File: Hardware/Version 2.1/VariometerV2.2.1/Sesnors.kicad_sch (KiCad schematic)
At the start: 19 parts, among them U4 DPS310, U5 BMI088, U6 QMC5883L, U7 MAX98357A

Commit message: Working on PCB
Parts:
- R36: footprint (none) -> Resistor_SMD:R_0603_1608Metric
- R41: footprint (none) -> Resistor_SMD:R_0805_2012Metric
- TP7, TP8, TP9: footprint (none) -> TestPoint:TestPoint_Pad_D1.5mm
- U4: footprint (none) -> MainLibrary:DPS310XTSA1
- U5: footprint (none) -> MainLibrary:BMI088
- U6: footprint (none) -> MainLibrary:QMC5883L
- U7: footprint (none) -> MainLibrary:QFN50P300X300X80-17N
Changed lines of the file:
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@@
       (effects (font (size 1.27 1.27)) (justify left))
     )
-    (property "Footprint" "" (at 71.12 143.51 0)
+    (property "Footprint" "TestPoint:TestPoint_Pad_D1.5mm" (at 71.12 143.51 0)
       (effects (font (size 1.27 1.27)) hide)
     )
@@
       (effects (font (size 1.27 1.27)))
     )
-    (property "Footprint" "" (at 60.96 52.07 0)
+    (property "Footprint" "MainLibrary:BMI088" (at 60.96 52.07 0)
       (effects (font (size 1.27 1.27)) hide)
     )
@@
       (effects (font (size 1.27 1.27)) (justify left))
     )
-    (property "Footprint" "" (at 66.04 143.51 0)
+    (property "Footprint" "TestPoint:TestPoint_Pad_D1.5mm" (at 66.04 143.51 0)
       (effects (font (size 1.27 1.27)) hide)
     )
@@
       (effects (font (size 1.27 1.27)) (justify left))
     )
-    (property "Footprint" "" (at 137.16 49.53 0)
+    (property "Footprint" "MainLibrary:QMC5883L" (at 137.16 49.53 0)
       (effects (font (size 1.27 1.27)) hide)
     )
@@
       (effects (font (size 1.27 1.27)))
     )
-    (property "Footprint" "" (at 231.14 39.37 0)
+    (property "Footprint" "MainLibrary:DPS310XTSA1" (at 231.14 39.37 0)
       (effects (font (size 1.27 1.27)) hide)
     )
@@
       (effects (font (size 1.27 1.27)) (justify left))
     )
-    (property "Footprint" "" (at 62.23 143.51 0)
+    (property "Footprint" "TestPoint:TestPoint_Pad_D1.5mm" (at 62.23 143.51 0)
       (effects (font (size 1.27 1.27)) hide)
     )
@@
       (effects (font (size 1.27 1.27)) (justify left))
     )
-    (property "Footprint" "" (at 31.75 157.48 0)
+    (property "Footprint" "Resistor_SMD:R_0805_2012Metric" (at 31.75 157.48 0)
       (effects (font (size 1.27 1.27)) hide)
     )
@@
       (effects (font (size 1.27 1.27)) (justify left))
     )
-    (property "Footprint" "" (at 214.63 44.45 0)
+    (property "Footprint" "Resistor_SMD:R_0603_1608Metric" (at 214.63 44.45 0)
       (effects (font (size 1.27 1.27)) hide)
     )
@@
       (effects (font (size 1.27 1.27)))
     )
-    (property "Footprint" "" (at 80.01 158.75 0)
-      (effects (font (size 1.27 1.27)) hide)
-    )
+    (property "Footprint" "MainLibrary:QFN50P300X300X80-17N" (at 80.01 158.75 0)
+      (effects (font (size 1.27 1.27)) hide)
+    )

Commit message: PCB
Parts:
- C35, C36, C37, C38, C39, C43: JLCPCB Part # C307331 -> (none); LCSC Part (none) -> C307331
- C40: JLCPCB Part # C19666 -> (none); LCSC Part (none) -> C19666
- C41: JLCPCB Part # C16772 -> (none); LCSC Part (none) -> C16772
- C42: JLCPCB Part # C96446 -> (none); LCSC Part (none) -> C19702
- R36: JLCPCB Part # C25741 -> (none); LCSC Part (none) -> C25803
- R41: LCSC Part (none) -> C17414
- U4: JLCPCB Part # C130156 -> (none); LCSC Part (none) -> C130156
- U5: JLCPCB Part # C194919 -> (none); LCSC Part (none) -> C194919
- U6: JLCPCB Part # C976032 -> (none); LCSC Part (none) -> C976032
- U7: JLCPCB Part # C910544 -> (none); LCSC Part (none) -> C910544
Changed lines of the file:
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@@
+      (effects (font (size 1.27 1.27)) hide)
+    )
+    (property "LCSC Part" "" (at 66.04 143.51 0)
       (effects (font (size 1.27 1.27)) hide)
     )
@@
       (effects (font (size 1.27 1.27)) hide)
     )
-    (property "JLCPCB Part #" "C194919" (at 60.96 52.07 0)
+    (property "LCSC Part" "C194919" (at 60.96 52.07 0)
       (effects (font (size 1.27 1.27)) hide)
     )
@@
       (effects (font (size 1.27 1.27)) hide)
     )
+    (property "LCSC Part" "" (at 60.96 143.51 0)
+      (effects (font (size 1.27 1.27)) hide)
+    )
     (pin "1")
     (instances
@@
       (effects (font (size 1.27 1.27)) hide)
     )
-    (property "JLCPCB Part #" "C976032" (at 137.16 49.53 0)
+    (property "LCSC Part" "C976032" (at 137.16 49.53 0)
       (effects (font (size 1.27 1.27)) hide)
     )
@@
       (effects (font (size 1.27 1.27)) hide)
     )
-    (property "JLCPCB Part #" "C96446" (at 38.1 171.45 0)
+    (property "LCSC Part" "C19702" (at 38.1 171.45 0)
       (effects (font (size 1.27 1.27)) hide)
     )
@@
       (effects (font (size 1.27 1.27)) hide)
     )
-    (property "JLCPCB Part #" "C307331" (at 49.53 171.45 0)
+    (property "LCSC Part" "C307331" (at 49.53 171.45 0)
       (effects (font (size 1.27 1.27)) hide)
     )
@@
       (effects (font (size 1.27 1.27)) hide)
     )
-    (property "JLCPCB Part #" "C307331" (at 256.54 46.99 0)
+    (property "LCSC Part" "C307331" (at 256.54 46.99 0)
       (effects (font (size 1.27 1.27)) hide)
     )
@@
       (effects (font (size 1.27 1.27)) hide)
     )
-    (property "JLCPCB Part #" "C307331" (at 55.88 31.75 0)
+    (property "LCSC Part" "C307331" (at 55.88 31.75 0)
       (effects (font (size 1.27 1.27)) hide)
     )
@@
       (effects (font (size 1.27 1.27)) hide)
     )
-    (property "JLCPCB Part #" "C19666" (at 134.62 76.2 0)
+    (property "LCSC Part" "C19666" (at 134.62 76.2 0)
       (effects (font (size 1.27 1.27)) hide)
     )
@@
       (effects (font (size 1.27 1.27)) hide)
     )
-    (property "JLCPCB Part #" "C130156" (at 231.14 39.37 0)
+    (property "LCSC Part" "C130156" (at 231.14 39.37 0)
       (effects (font (size 1.27 1.27)) hide)
     )
@@
       (effects (font (size 1.27 1.27)) hide)
     )
+    (property "LCSC Part" "" (at 110.49 158.75 0)
+      (effects (font (size 1.27 1.27)) hide)
+    )
     (pin "1")
     (pin "2")
@@
       (effects (font (size 1.27 1.27)) hide)
     )
-    (property "JLCPCB Part #" "C307331" (at 128.27 35.56 0)
+    (property "LCSC Part" "C307331" (at 128.27 35.56 0)
       (effects (font (size 1.27 1.27)) hide)
     )
@@
       (effects (font (size 1.27 1.27)) hide)
     )
+    (property "LCSC Part" "" (at 57.15 143.51 0)
+      (effects (font (size 1.27 1.27)) hide)
+    )
     (pin "1")
     (instances
@@
       (effects (font (size 1.27 1.27)) hide)
     )
-    (property "JLCPCB Part #" "C307331" (at 73.66 31.75 0)
+    (property "LCSC Part" "C307331" (at 73.66 31.75 0)
       (effects (font (size 1.27 1.27)) hide)
     )
@@
       (effects (font (size 1.27 1.27)) hide)
     )
-    (property "JLCPCB Part #" "C16772" (at 153.67 52.07 0)
+    (property "LCSC Part" "C16772" (at 153.67 52.07 0)
       (effects (font (size 1.27 1.27)) hide)
     )
@@
       (effects (font (size 1.27 1.27)) hide)
     )
+    (property "LCSC Part" "C17414" (at 31.75 157.48 0)
+      (effects (font (size 1.27 1.27)) hide)
+    )
     (pin "1")
     (pin "2")
@@
       (effects (font (size 1.27 1.27)) hide)
     )
-    (property "JLCPCB Part #" "C25741" (at 214.63 44.45 0)
+    (property "LCSC Part" "C25803" (at 214.63 44.45 0)
       (effects (font (size 1.27 1.27)) hide)
     )
@@
       (effects (font (size 1.27 1.27)) hide)
     )
-    (property "JLCPCB Part #" "C910544" (at 80.01 158.75 0)
+    (property "LCSC Part" "C910544" (at 80.01 158.75 0)
       (effects (font (size 1.27 1.27)) hide)
     )
@@
       (effects (font (size 1.27 1.27)) hide)
     )
-    (property "JLCPCB Part #" "C307331" (at 250.19 34.29 0)
-      (effects (font (size 1.27 1.27)) hide)
-    )
+    (property "LCSC Part" "C307331" (at 250.19 34.29 0)
+      (effects (font (size 1.27 1.27)) hide)
+    )

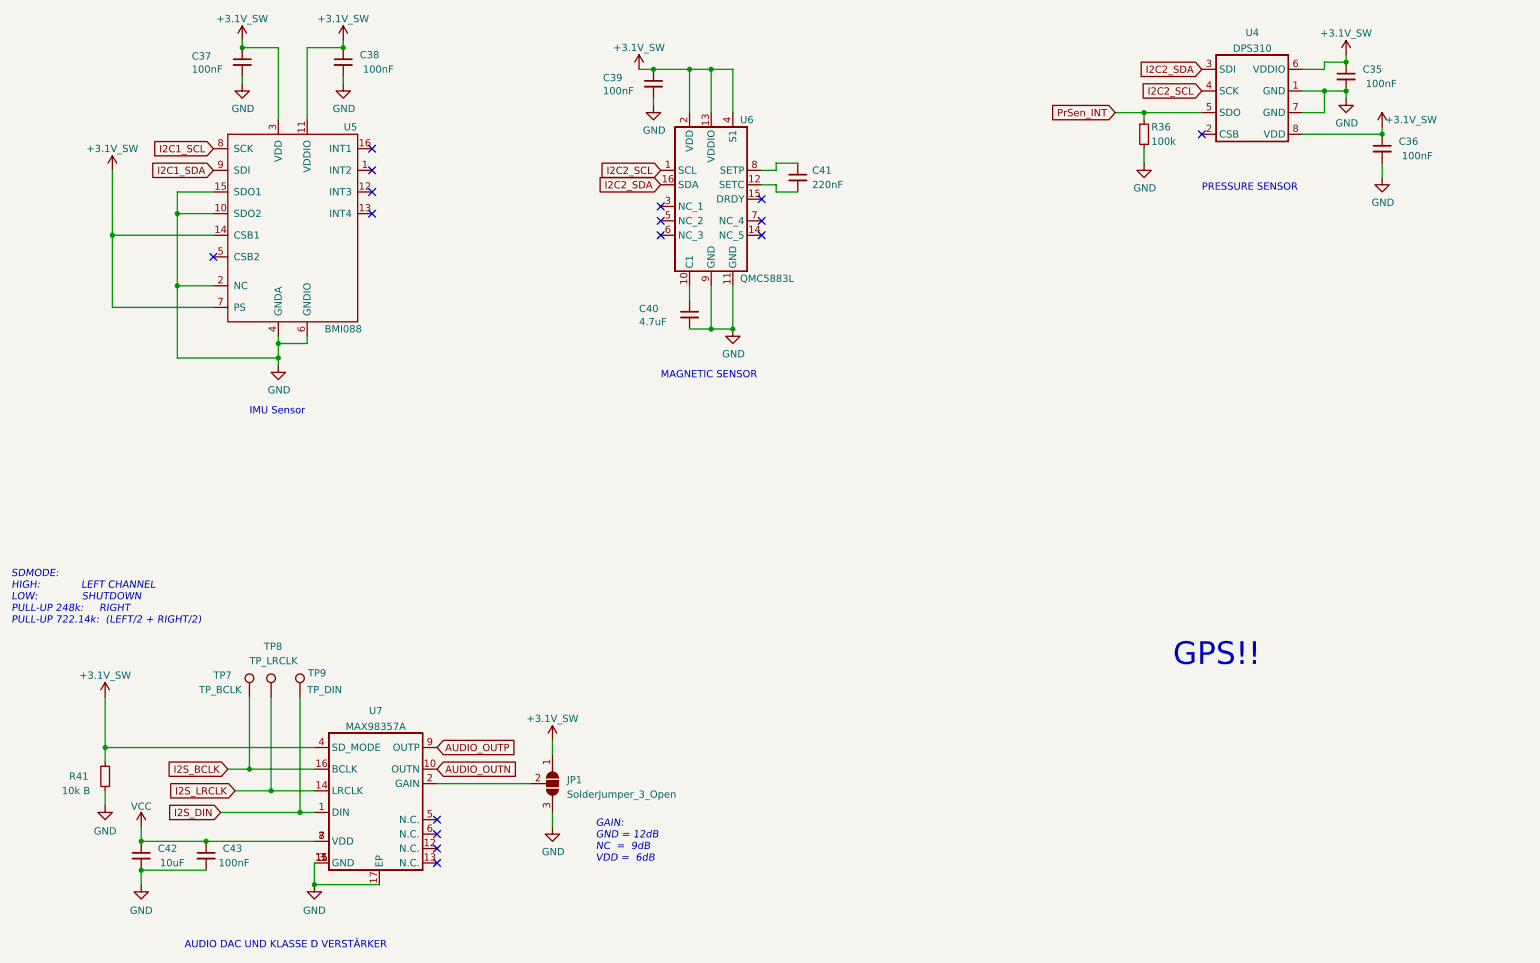
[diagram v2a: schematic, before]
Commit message: Start on pcb
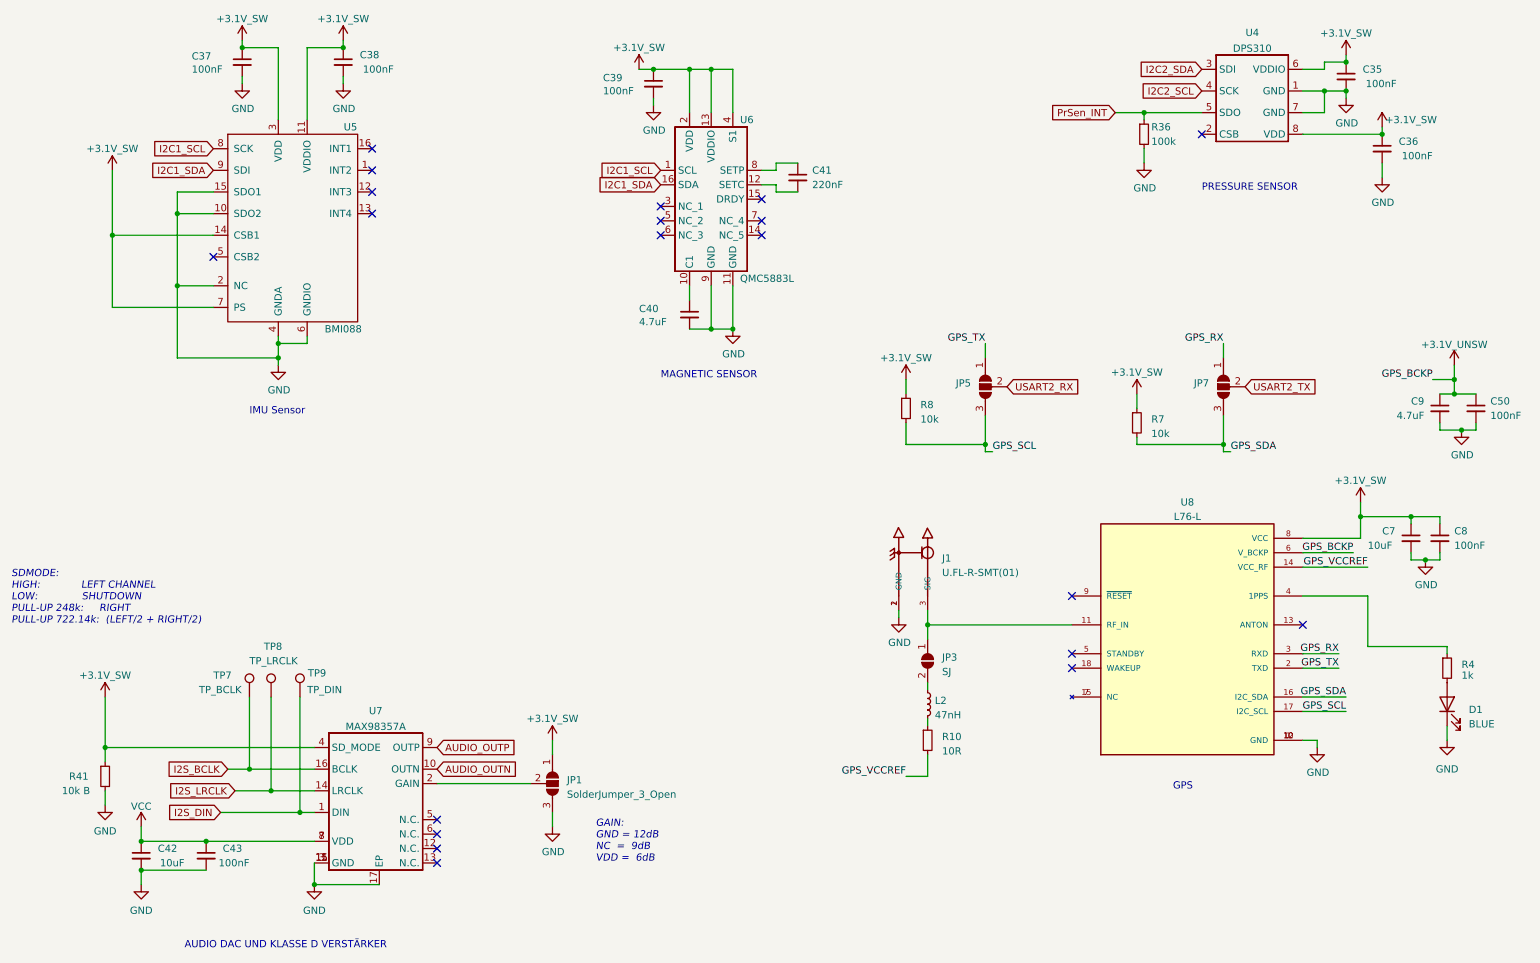
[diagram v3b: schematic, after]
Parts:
- added C50, C8: 100nF, Capacitor_SMD:C_0402_1005Metric, symbol Device:C_Small
- added C7: 10uF, Capacitor_SMD:C_0402_1005Metric, symbol Device:C_Small
- added C9: 4.7uF, Capacitor_SMD:C_0402_1005Metric, symbol Device:C_Small
- added D1: BLUE, LED_SMD:LED_0603_1608Metric, symbol Device:LED
- added J1: U.FL-R-SMT(01), SamacSys_Parts:HRS_U.FL-R-SMT(01), symbol Main_Library:U.FL-R-SMT(01)
- added JP3: SJ, Jumper:SolderJumper-2_P1.3mm_Open_Pad1.0x1.5mm, symbol Jumper:SolderJumper_2_Open
- added JP5, JP7: ~, Jumper:SolderJumper-3_P1.3mm_Open_Pad1.0x1.5mm, symbol Jumper:SolderJumper_3_Open
- added L2: 47nH, Inductor_SMD:L_0805_2012Metric, symbol Device:L_Small
- added R10: 10R, Resistor_SMD:R_0603_1608Metric, symbol Device:R_Small
- added R4: 1k, Resistor_SMD:R_0603_1608Metric, symbol Device:R_Small
- added R7: 10k, Inductor_SMD:L_0603_1608Metric, symbol Device:R_Small
- added R8: 10k, Resistor_SMD:R_0603_1608Metric, symbol Device:R_Small
- added U8: L76-L, MainLibrary:XCVR_L76-L, symbol Main_LibraryVario:L76-L
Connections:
- net +3.1V_SW: now also C7.1, C8.1, R7.1, R8.1, U8.8 (VCC)
- net GND: now also C50.2, C7.2, C8.2, C9.2, D1.1 (K), J1.1 (GND), J1.2 (GND), U8.1 (GND), U8.10 (GND), U8.12 (GND)
- net I2C1_SCL: now also U6.1 (SCL)
- net I2C1_SDA: now also U6.16 (SDA)
- net I2C2_SCL: no longer U6.1 (SCL)
- net I2C2_SDA: no longer U6.16 (SDA)
- new net: JP3.2 (B), L2.1
- new net: L2.2, R10.1
- new net: D1.2 (A), R4.2
- new net: J1.3 (SIG), JP3.1 (A), U8.11 (RF_IN)
- new net: U8.15 (NC), U8.7 (NC)
- new net: R4.1, U8.4 (1PPS)
- new net +3.1V_UNSW: C50.1, C9.1, U8.6 (V_BCKP)
- new net GPS_RX: JP7.1 (A), U8.3 (RXD)
- new net GPS_SCL: JP5.3 (B), R8.2, U8.17 (I2C_SCL)
- new net GPS_SDA: JP7.3 (B), R7.2, U8.16 (I2C_SDA)
- new net GPS_TX: JP5.1 (A), U8.2 (TXD)
- new net GPS_VCCREF: R10.2, U8.14 (VCC_RF)
- new net USART2_RX: JP5.2 (C)
- new net USART2_TX: JP7.2 (C)
- no-connect marks 16 -> 20
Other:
- note added: "GPS"
- note removed: "GPS!!"
